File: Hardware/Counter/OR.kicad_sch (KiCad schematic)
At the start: 6 parts, among them Q125 FDN335N, Q126 FDN360P, Q127 FDN335N, Q128 FDN335N, U70 FDN360P, U71 FDN360P

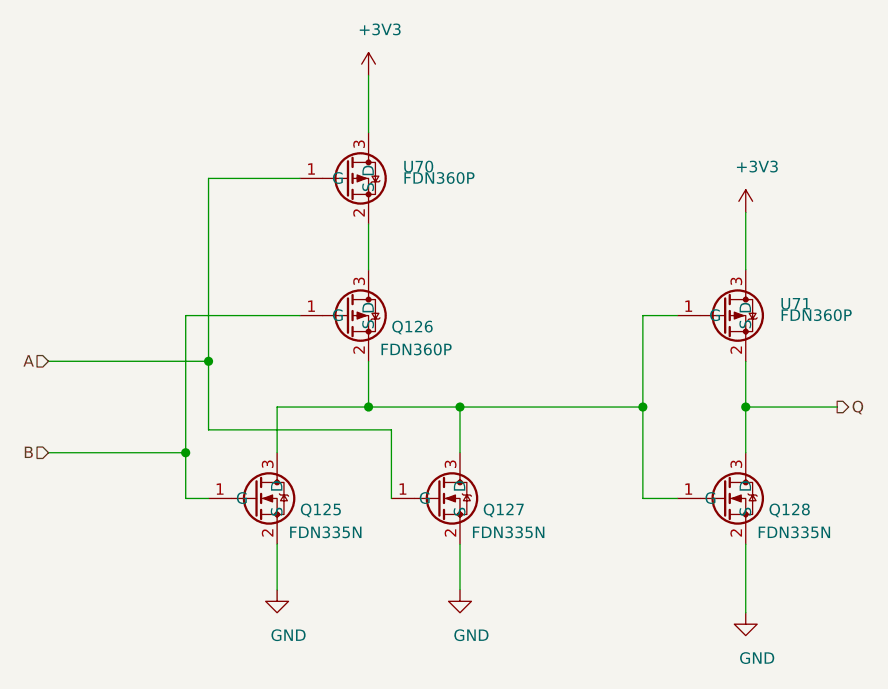
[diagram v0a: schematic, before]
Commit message: working on connectin bits together
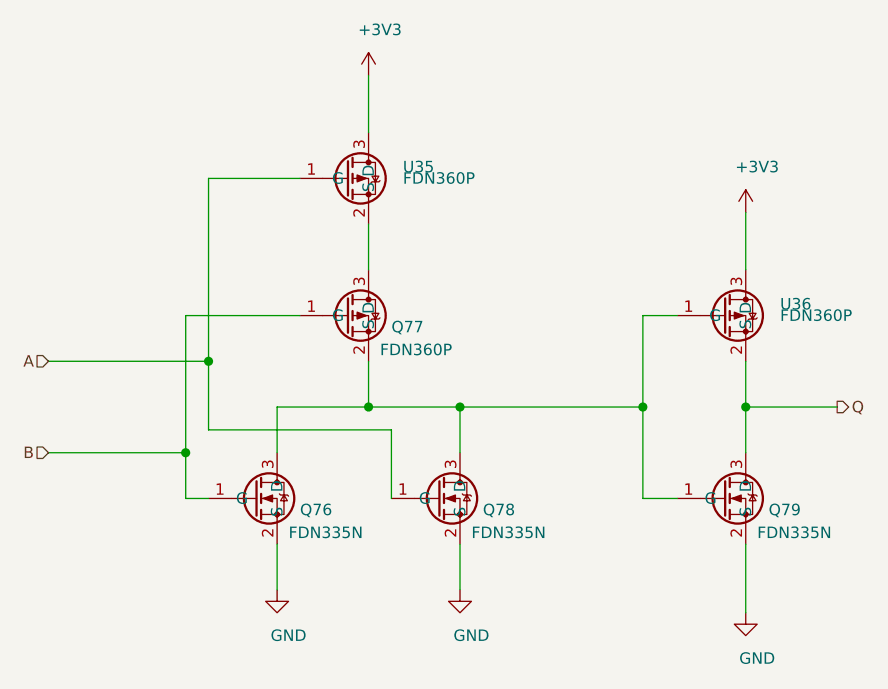
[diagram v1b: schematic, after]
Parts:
- renumbered Q125 to Q76, Q126 to Q77, Q127 to Q78, Q128 to Q79, U70 to U35, U71 to U36
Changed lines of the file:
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@@
   (symbol (lib_id "power:+3V3") (at 138.43 57.15 0)
     (in_bom yes) (on_board yes)
-    (property "Reference" "#PWR0254" (id 0) (at 138.43 60.96 0)
+    (property "Reference" "#PWR0197" (id 0) (at 138.43 60.96 0)
       (effects (font (size 1.27 1.27)) hide)
     )
@@
   (symbol (lib_id "power:+3V3") (at 180.34 72.39 0)
     (in_bom yes) (on_board yes)
-    (property "Reference" "#PWR0256" (id 0) (at 180.34 76.2 0)
+    (property "Reference" "#PWR0199" (id 0) (at 180.34 76.2 0)
       (effects (font (size 1.27 1.27)) hide)
     )
@@
   (symbol (lib_id "power:GND") (at 128.27 114.3 0)
     (in_bom yes) (on_board yes)
-    (property "Reference" "#PWR0252" (id 0) (at 128.27 120.65 0)
+    (property "Reference" "#PWR0195" (id 0) (at 128.27 120.65 0)
       (effects (font (size 1.27 1.27)) hide)
     )
@@
   (symbol (lib_id "power:GND") (at 148.59 114.3 0)
     (in_bom yes) (on_board yes)
-    (property "Reference" "#PWR0253" (id 0) (at 148.59 120.65 0)
+    (property "Reference" "#PWR0196" (id 0) (at 148.59 120.65 0)
       (effects (font (size 1.27 1.27)) hide)
     )
@@
   (symbol (lib_id "power:GND") (at 180.34 116.84 0)
     (in_bom yes) (on_board yes)
-    (property "Reference" "#PWR0255" (id 0) (at 180.34 123.19 0)
+    (property "Reference" "#PWR0198" (id 0) (at 180.34 123.19 0)
       (effects (font (size 1.27 1.27)) hide)
     )
@@
   (symbol (lib_id "Custom_Transistors:FDN335N") (at 128.27 104.14 0)
     (in_bom yes) (on_board yes)
-    (property "Reference" "Q125" (id 0) (at 130.81 105.41 0)
+    (property "Reference" "Q76" (id 0) (at 130.81 105.41 0)
       (effects (font (size 1.27 1.27)) (justify left))
     )
@@
   (symbol (lib_name "Custom_Transistors:FDN360P_1") (lib_id "Custom_Transistors:FDN360P") (at 138.43 68.58 0)
     (in_bom yes) (on_board yes)
-    (property "Reference" "U70" (id 0) (at 142.24 67.31 0)
+    (property "Reference" "U35" (id 0) (at 142.24 67.31 0)
       (effects (font (size 1.27 1.27)) (justify left))
     )
@@
   (symbol (lib_name "Custom_Transistors:FDN360P_2") (lib_id "Custom_Transistors:FDN360P") (at 138.43 83.82 0)
     (in_bom yes) (on_board yes)
-    (property "Reference" "Q126" (id 0) (at 140.97 85.09 0)
+    (property "Reference" "Q77" (id 0) (at 140.97 85.09 0)
       (effects (font (size 1.27 1.27)) (justify left))
     )
@@
   (symbol (lib_id "Custom_Transistors:FDN335N") (at 148.59 104.14 0)
     (in_bom yes) (on_board yes)
-    (property "Reference" "Q127" (id 0) (at 151.13 105.41 0)
+    (property "Reference" "Q78" (id 0) (at 151.13 105.41 0)
       (effects (font (size 1.27 1.27)) (justify left))
     )
@@
   (symbol (lib_id "Custom_Transistors:FDN360P") (at 180.34 83.82 0)
     (in_bom yes) (on_board yes)
-    (property "Reference" "U71" (id 0) (at 184.15 82.55 0)
+    (property "Reference" "U36" (id 0) (at 184.15 82.55 0)
       (effects (font (size 1.27 1.27)) (justify left))
     )
@@
   (symbol (lib_id "Custom_Transistors:FDN335N") (at 180.34 104.14 0)
     (in_bom yes) (on_board yes)
-    (property "Reference" "Q128" (id 0) (at 182.88 105.41 0)
+    (property "Reference" "Q79" (id 0) (at 182.88 105.41 0)
       (effects (font (size 1.27 1.27)) (justify left))
     )

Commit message: kicad updates
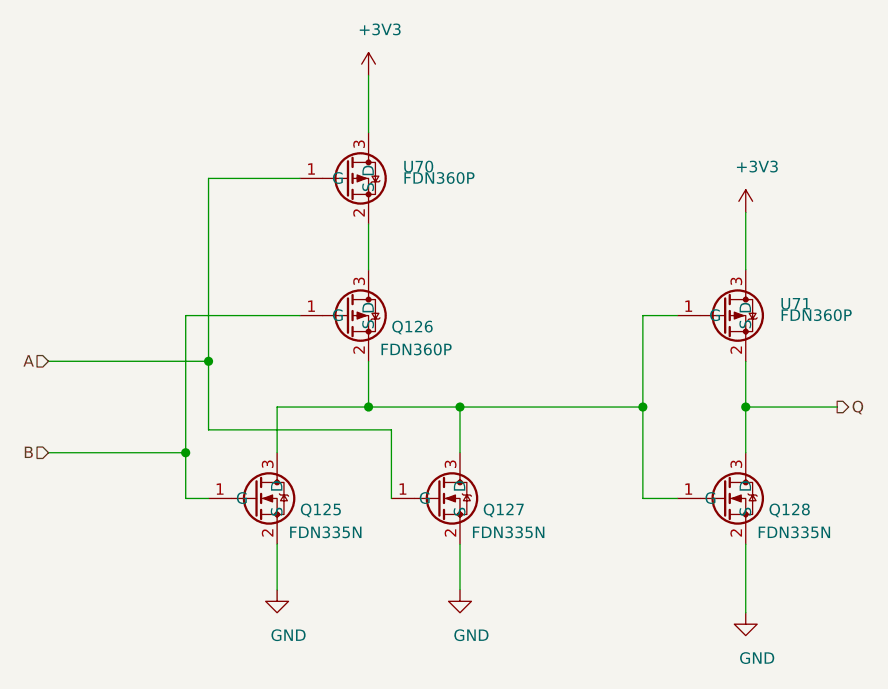
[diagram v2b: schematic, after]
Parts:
- renumbered Q76 to Q125, Q77 to Q126, Q78 to Q127, Q79 to Q128, U35 to U70, U36 to U71
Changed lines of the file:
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@@
   (symbol (lib_id "power:+3V3") (at 138.43 57.15 0)
     (in_bom yes) (on_board yes)
-    (property "Reference" "#PWR0197" (id 0) (at 138.43 60.96 0)
+    (property "Reference" "#PWR0254" (id 0) (at 138.43 60.96 0)
       (effects (font (size 1.27 1.27)) hide)
     )
@@
   (symbol (lib_id "power:+3V3") (at 180.34 72.39 0)
     (in_bom yes) (on_board yes)
-    (property "Reference" "#PWR0199" (id 0) (at 180.34 76.2 0)
+    (property "Reference" "#PWR0256" (id 0) (at 180.34 76.2 0)
       (effects (font (size 1.27 1.27)) hide)
     )
@@
   (symbol (lib_id "power:GND") (at 128.27 114.3 0)
     (in_bom yes) (on_board yes)
-    (property "Reference" "#PWR0195" (id 0) (at 128.27 120.65 0)
+    (property "Reference" "#PWR0252" (id 0) (at 128.27 120.65 0)
       (effects (font (size 1.27 1.27)) hide)
     )
@@
   (symbol (lib_id "power:GND") (at 148.59 114.3 0)
     (in_bom yes) (on_board yes)
-    (property "Reference" "#PWR0196" (id 0) (at 148.59 120.65 0)
+    (property "Reference" "#PWR0253" (id 0) (at 148.59 120.65 0)
       (effects (font (size 1.27 1.27)) hide)
     )
@@
   (symbol (lib_id "power:GND") (at 180.34 116.84 0)
     (in_bom yes) (on_board yes)
-    (property "Reference" "#PWR0198" (id 0) (at 180.34 123.19 0)
+    (property "Reference" "#PWR0255" (id 0) (at 180.34 123.19 0)
       (effects (font (size 1.27 1.27)) hide)
     )
@@
   (symbol (lib_id "Custom_Transistors:FDN335N") (at 128.27 104.14 0)
     (in_bom yes) (on_board yes)
-    (property "Reference" "Q76" (id 0) (at 130.81 105.41 0)
+    (property "Reference" "Q125" (id 0) (at 130.81 105.41 0)
       (effects (font (size 1.27 1.27)) (justify left))
     )
@@
   (symbol (lib_name "Custom_Transistors:FDN360P_1") (lib_id "Custom_Transistors:FDN360P") (at 138.43 68.58 0)
     (in_bom yes) (on_board yes)
-    (property "Reference" "U35" (id 0) (at 142.24 67.31 0)
+    (property "Reference" "U70" (id 0) (at 142.24 67.31 0)
       (effects (font (size 1.27 1.27)) (justify left))
     )
@@
   (symbol (lib_name "Custom_Transistors:FDN360P_2") (lib_id "Custom_Transistors:FDN360P") (at 138.43 83.82 0)
     (in_bom yes) (on_board yes)
-    (property "Reference" "Q77" (id 0) (at 140.97 85.09 0)
+    (property "Reference" "Q126" (id 0) (at 140.97 85.09 0)
       (effects (font (size 1.27 1.27)) (justify left))
     )
@@
   (symbol (lib_id "Custom_Transistors:FDN335N") (at 148.59 104.14 0)
     (in_bom yes) (on_board yes)
-    (property "Reference" "Q78" (id 0) (at 151.13 105.41 0)
+    (property "Reference" "Q127" (id 0) (at 151.13 105.41 0)
       (effects (font (size 1.27 1.27)) (justify left))
     )
@@
   (symbol (lib_id "Custom_Transistors:FDN360P") (at 180.34 83.82 0)
     (in_bom yes) (on_board yes)
-    (property "Reference" "U36" (id 0) (at 184.15 82.55 0)
+    (property "Reference" "U71" (id 0) (at 184.15 82.55 0)
       (effects (font (size 1.27 1.27)) (justify left))
     )
@@
   (symbol (lib_id "Custom_Transistors:FDN335N") (at 180.34 104.14 0)
     (in_bom yes) (on_board yes)
-    (property "Reference" "Q79" (id 0) (at 182.88 105.41 0)
+    (property "Reference" "Q128" (id 0) (at 182.88 105.41 0)
       (effects (font (size 1.27 1.27)) (justify left))
     )
